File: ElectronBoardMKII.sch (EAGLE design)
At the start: 54 parts, among them IC1 7805TV, K1 AQYAQY27, Q1 BSS170, Q2 BSS170, U1 LM386N

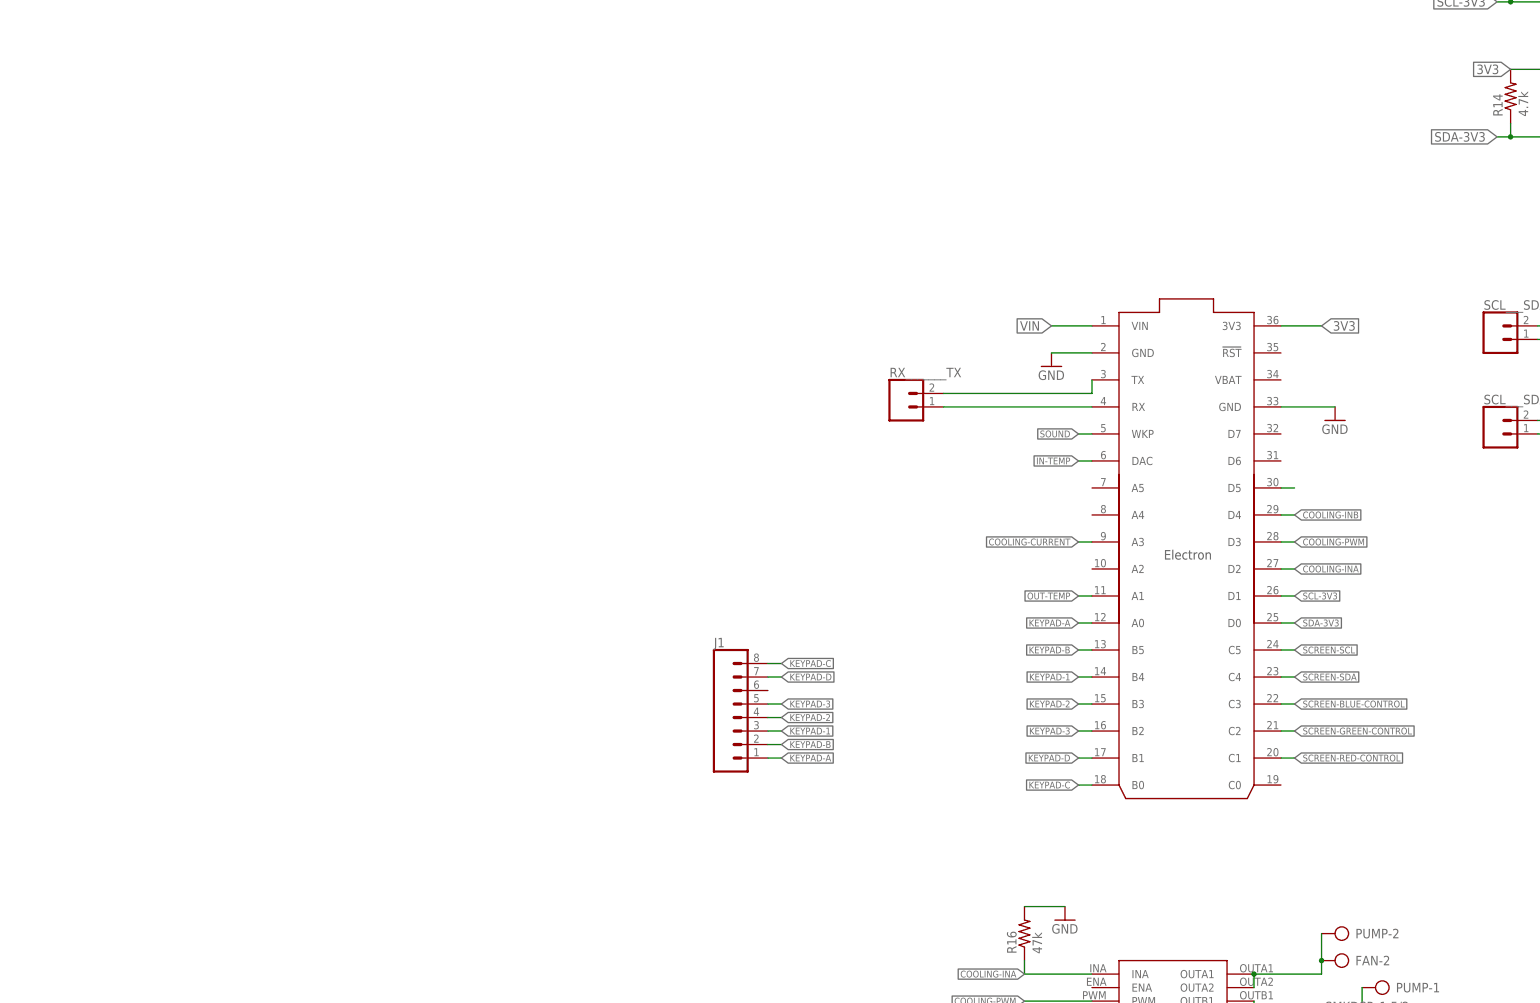
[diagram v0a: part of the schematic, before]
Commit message: Electron Side Header Start
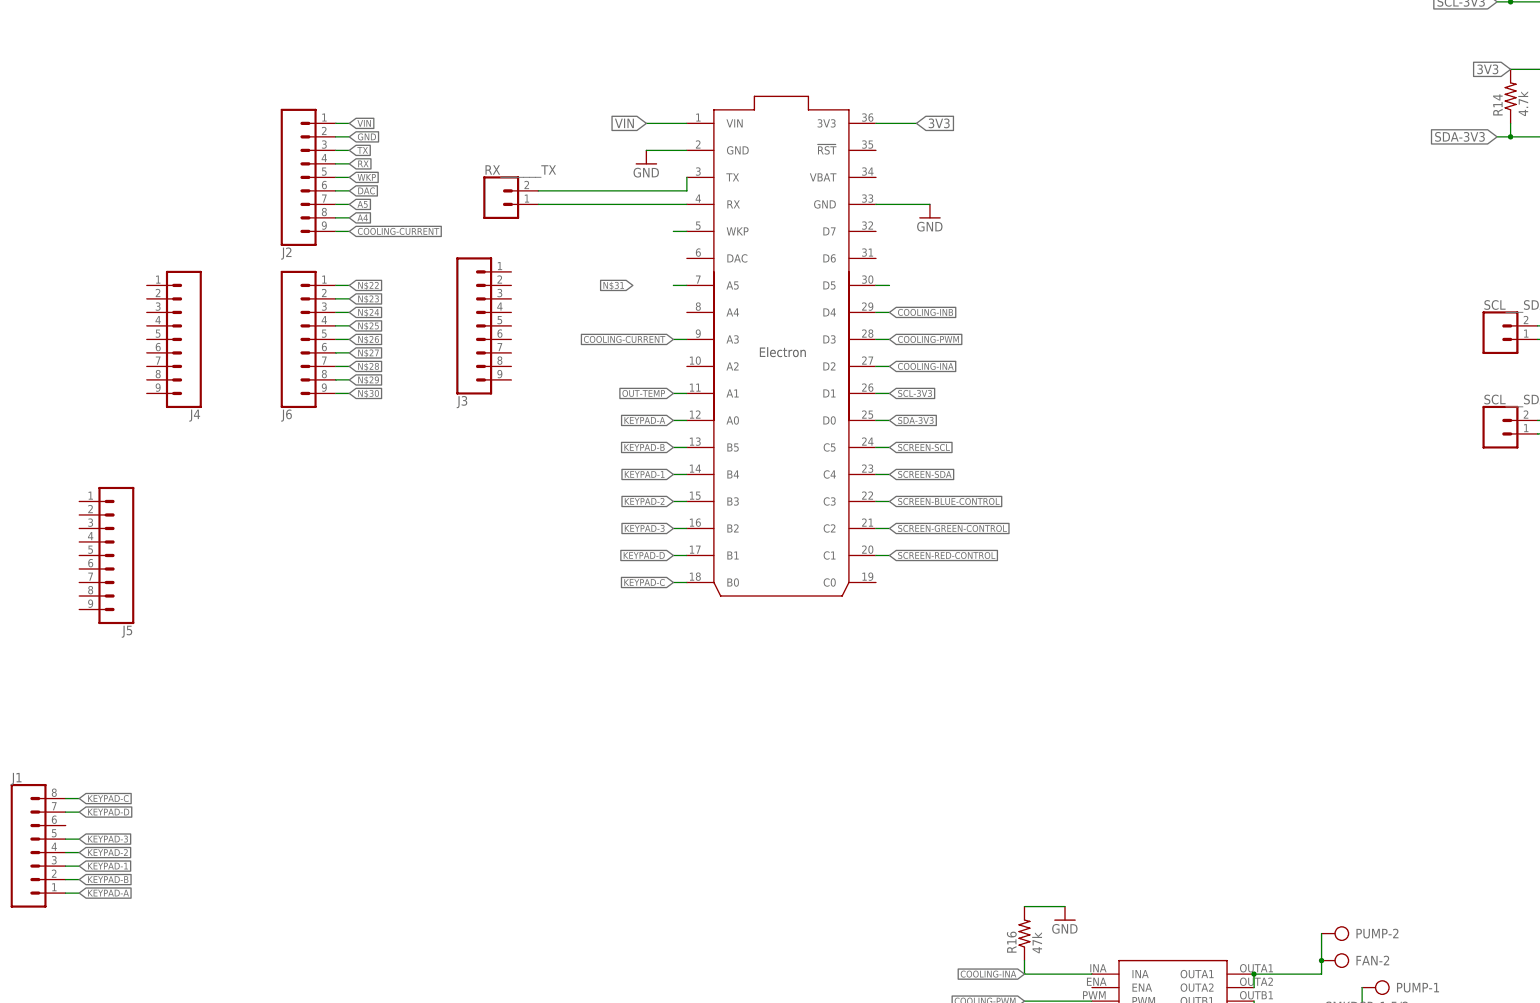
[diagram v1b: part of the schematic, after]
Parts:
- added J2, J3, J4, J5, J6: (no value), SparkFun-Connectors:CONN_09LOCK
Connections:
- new net A4: J2.8
- new net A5: J2.7
- new net DAC: J2.6
- new net N$22: J6.1
- new net N$23: J6.2
- new net N$24: J6.3
- new net N$25: J6.4
- new net N$26: J6.5
- new net N$27: J6.6
- new net N$28: J6.7
- new net N$29: J6.8
- new net N$30: J6.9
- new net N$31: U$1.A5
- new net WKP: J2.5
- net COOLING-CURRENT: now also J2.9
- net GND: now also J2.2
- net IN-TEMP: no longer U$1.DAC
- net RX: now also J2.4
- net TX: now also J2.3
- net VIN: now also J2.1
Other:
- moved on the sheet: J1, RX_______TX
